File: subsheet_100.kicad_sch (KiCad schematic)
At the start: 16 parts, among them J4 RS-232, U11 MC68901_DIP_48_PHY, U13 1489_SOCKET, U14 1488_PHY, Y1 2.4576 MHz

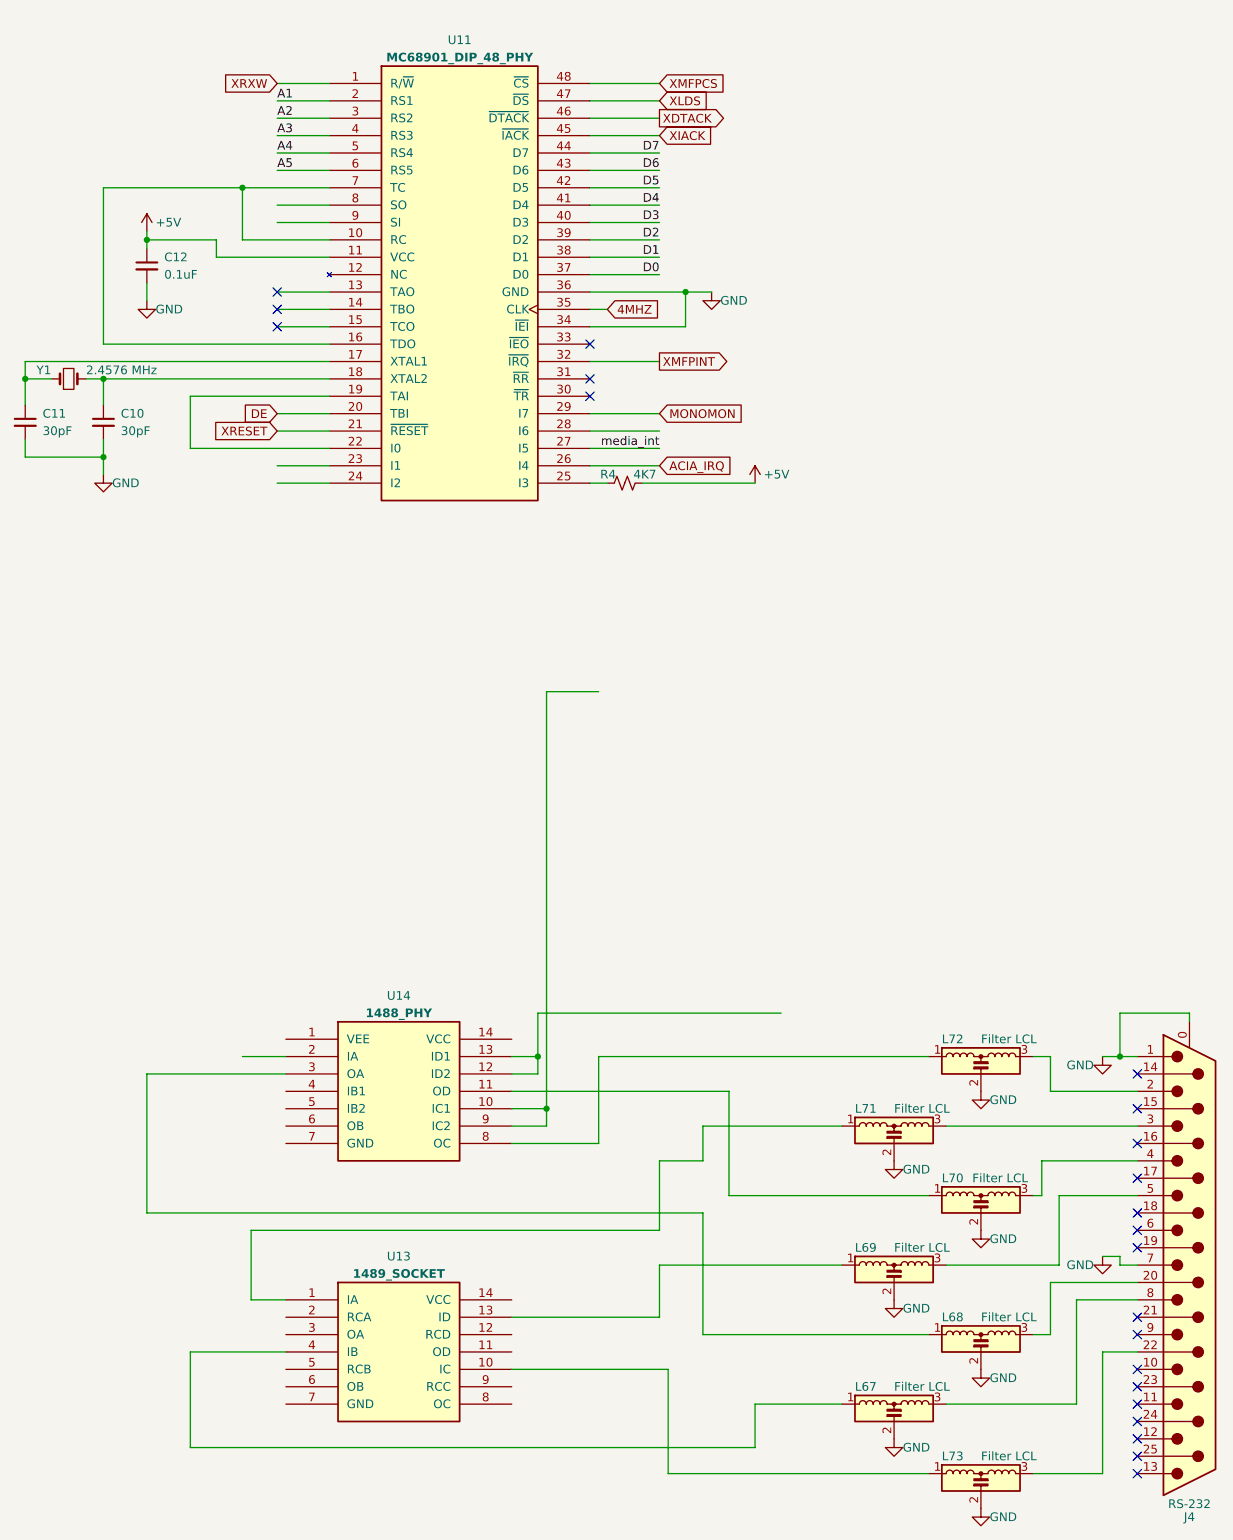
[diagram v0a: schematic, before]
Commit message: done RS-232 port to MFP68901
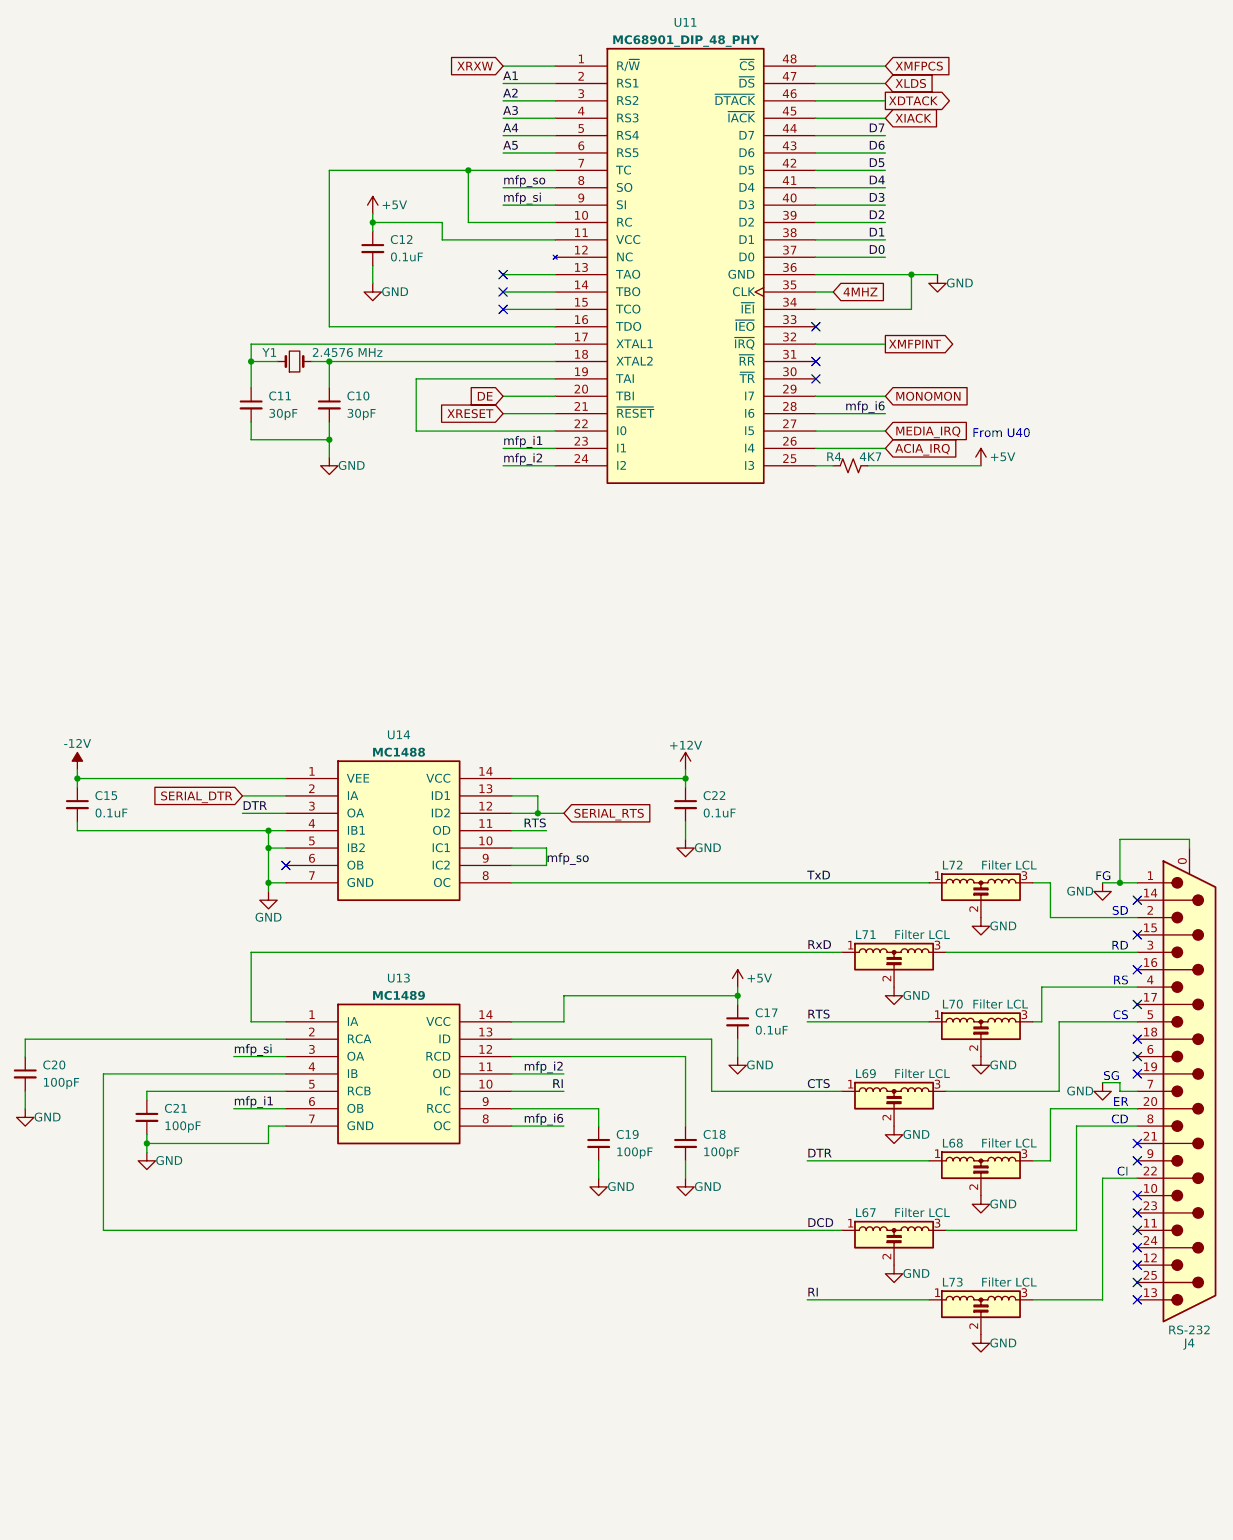
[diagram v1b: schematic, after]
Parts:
- added C15, C17, C22: 0.1uF, commons-passives_THT:Passive_THT_capacitor_mlcc_W2.54mm_L12.70mm, symbol Device:C_Small
- added C18, C19, C20, C21: 100pF, commons-passives_THT:Passive_THT_capacitor_mlcc_W2.54mm_L12.70mm, symbol Device:C_Small
- U13: value 1489_SOCKET -> MC1489; symbol mc1489:1489_SOCKET -> mc1489:1489_PHY
- U14: value 1488_PHY -> MC1488
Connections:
- net +5V: now also U13.14 (VCC), C17.1
- net GND: now also U13.7 (GND), U14.4 (IB1), U14.5 (IB2), U14.7 (GND), C15.2, C17.2, C18.2, C19.2, C20.2, C21.2, C22.2
- net RI: now reaches L73.1, U13.10 (IC)
- net RxD: now reaches L71.1, U13.1 (IA)
- net RTS: now reaches L70.1, U14.11 (OD)
- net CTS: now reaches L69.1, U13.13 (ID)
- net DTR: now reaches L68.1, U14.3 (OA)
- net DCD: now reaches L67.1, U13.4 (IB)
- net TxD: now reaches L72.1, U14.8 (OC)
- net mfp_i1: now reaches U11.23 (I1)
- net mfp_i1: now also U13.6 (OB)
- net mfp_i2: now reaches U11.24 (I2)
- net mfp_i2: now also U13.11 (OD)
- net mfp_i6: now reaches U11.28 (I6)
- net mfp_i6: now also U13.8 (OC)
- net mfp_so: now reaches U11.8 (SO)
- net mfp_so: now also U14.10 (IC1), U14.9 (IC2)
- net mfp_si: now reaches U11.9 (SI)
- net mfp_si: now also U13.3 (OA)
- net at U13.12 (RCD): now also C18.1
- net at U13.2 (RCA): now also C20.1
- net at U13.5 (RCB): now also C21.1
- net at U13.9 (RCC): now also C19.1
- net -12V: now reaches U14.1 (VEE)
- net -12V: now also C15.1
- net SERIAL_RTS: now reaches U14.12 (ID2), U14.13 (ID1)
- net +12V: now reaches U14.14 (VCC)
- net +12V: now also C22.1
- net SERIAL_DTR: now reaches U14.2 (IA)
- net media_int renamed MEDIA_IRQ
- no-connect marks 22 -> 23
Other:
- note added: "CD"
- note added: "CI"
- note added: "CS"
- note added: "ER"
- note added: "FG"
- note added: "From U40"
- note added: "RD"
- note added: "RS"
- note added: "SD"
- note added: "SG"
- moved on the sheet: C10, C11, C12, J4, L67, L68, L69, L70, L71, L72, L73, R4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
